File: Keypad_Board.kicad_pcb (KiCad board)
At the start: 2 copper layers, 45 x 62 mm, 40 parts, among them IC1 STM32L010K4T6, IC2 TMUX136RSER, J3 Data_Conn, J4 SEL Jumper, J5 SW_Header, J6 BOOT Jumper

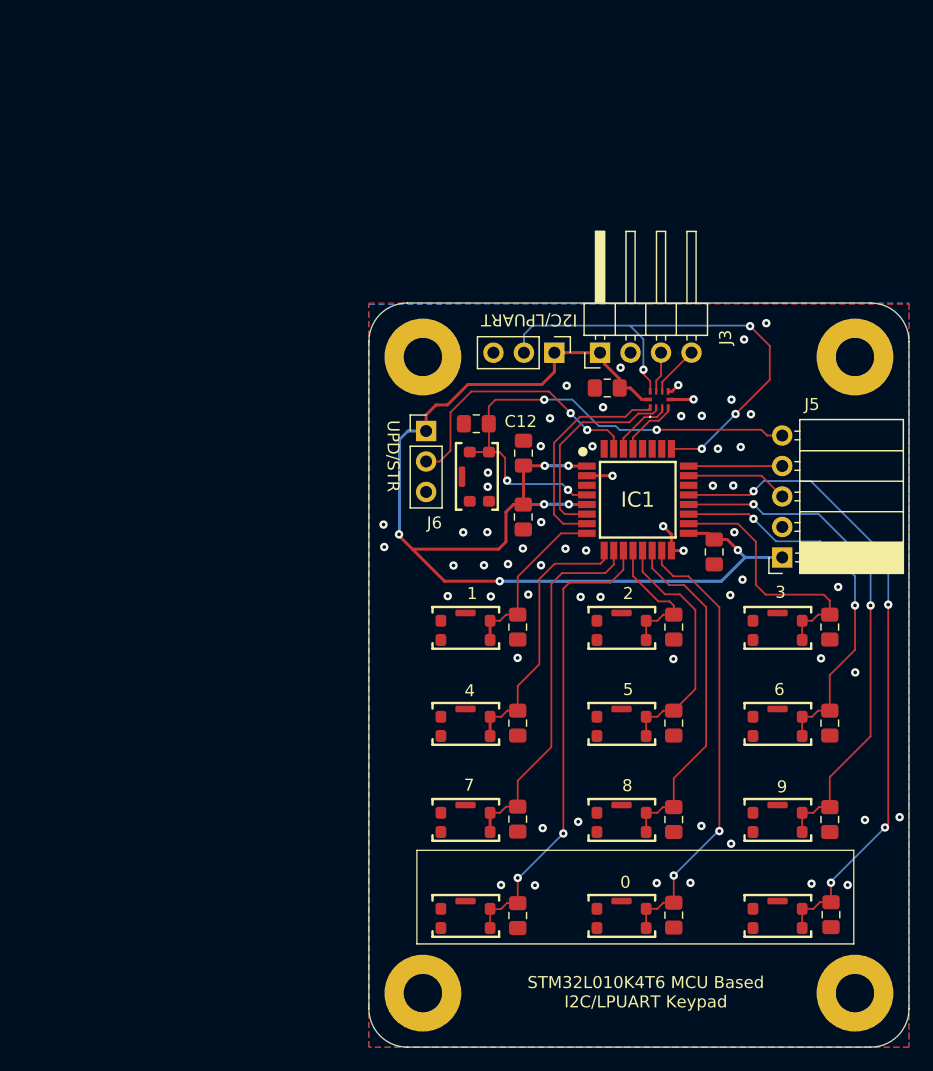
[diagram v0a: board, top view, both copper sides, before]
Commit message: Update
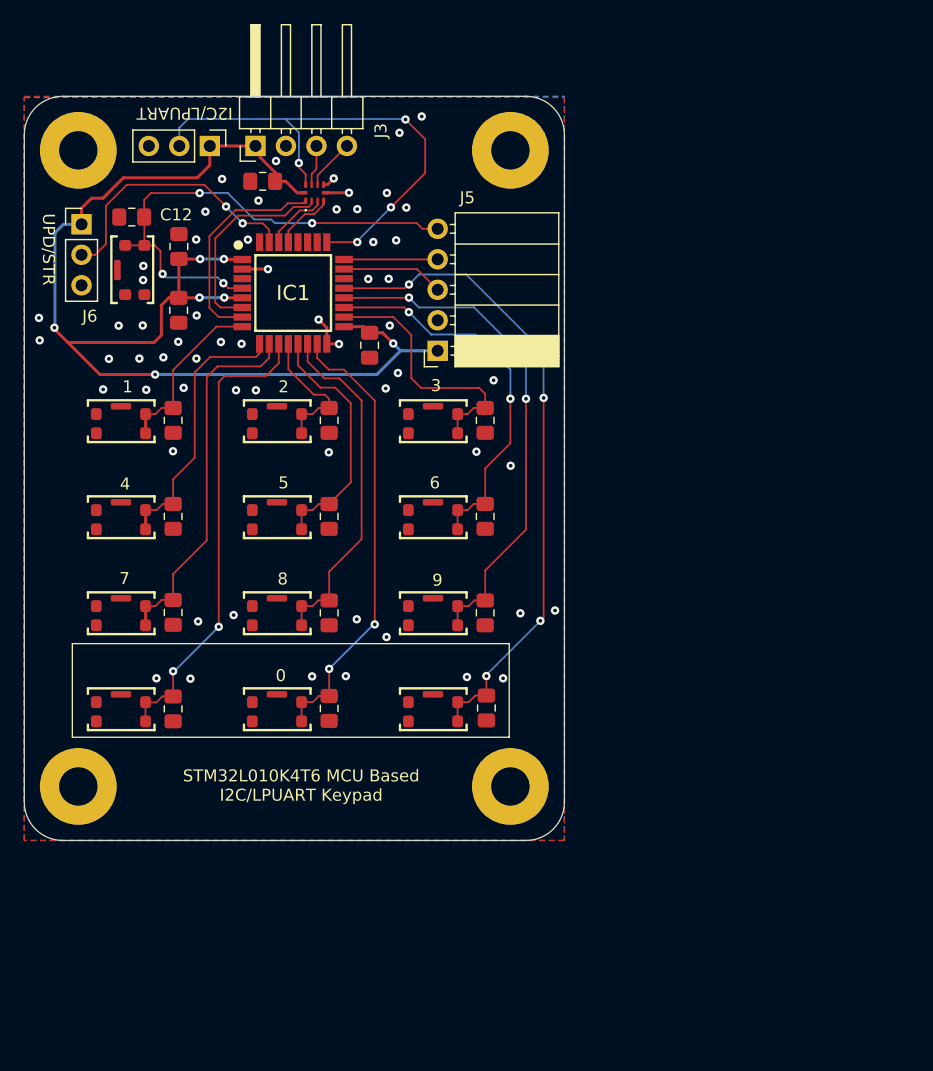
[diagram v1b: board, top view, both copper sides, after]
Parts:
- moved C12 33.5 mm to (90.2, 41.8)
- moved C13 33.5 mm to (93.7, 58.8)
- moved C14 33.5 mm to (101.2, 38.9)
- moved C15 33.5 mm to (93.7, 66.8)
- moved C16 33.5 mm to (93.7, 74.8)
- moved C17 33.5 mm to (93.7, 82.8)
- moved C18 33.5 mm to (106.7, 58.8)
- moved C19 33.5 mm to (106.7, 66.8)
- moved C20 33.5 mm to (106.7, 74.8)
- moved C21 33.5 mm to (106.7, 82.8)
- moved C22 33.5 mm to (119.7, 58.8)
- moved C23 33.5 mm to (119.7, 66.8)
- moved C24 33.5 mm to (119.7, 74.8)
- moved U14 33.5 mm to (99.8, 60.4)
- moved U15 33.5 mm to (99.8, 68.4)
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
